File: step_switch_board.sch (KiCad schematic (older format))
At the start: 37 parts

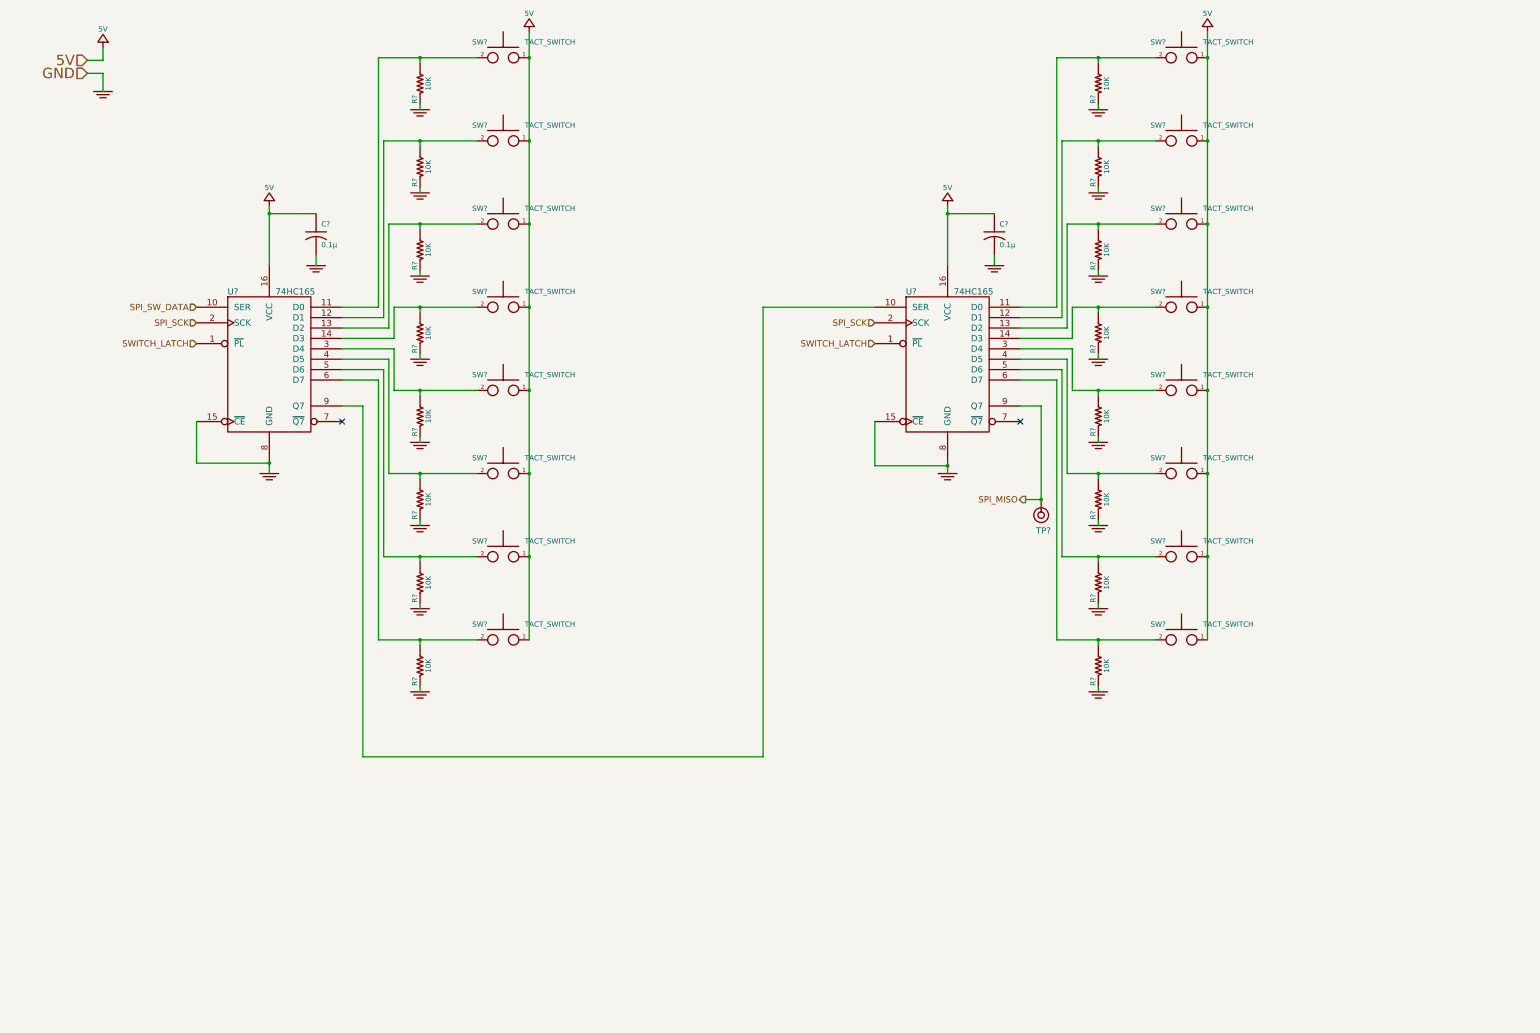
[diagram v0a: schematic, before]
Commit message: more SPI work
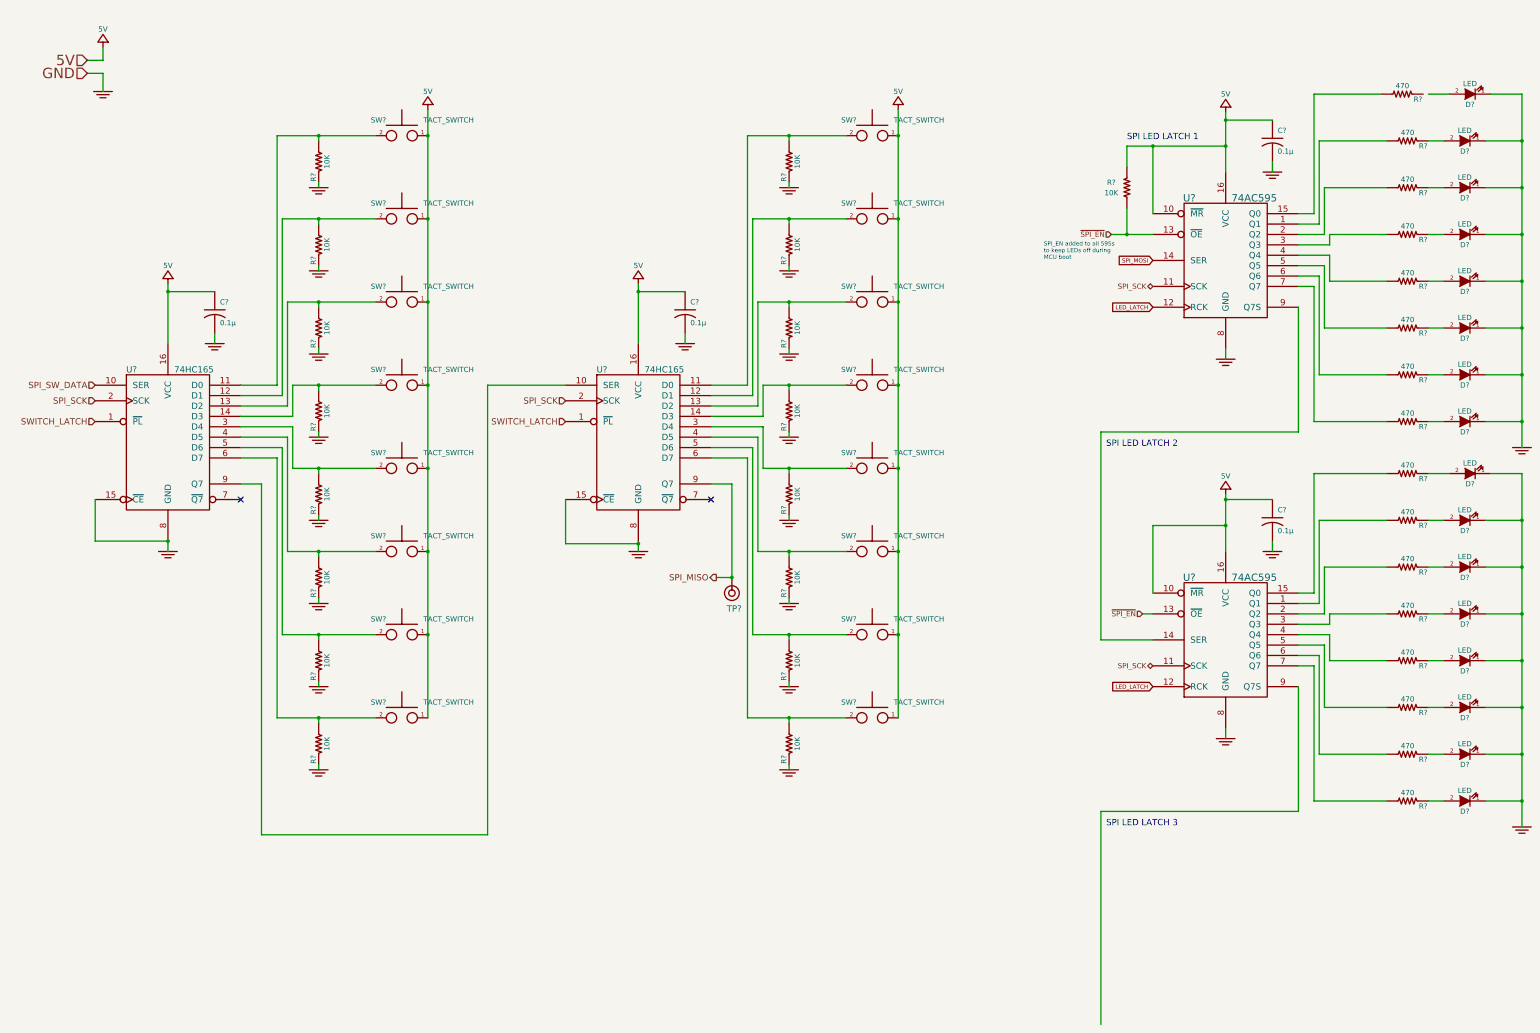
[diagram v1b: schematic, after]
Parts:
- added C? (x2): 0.1µ, ~, symbol C_US
- added D? (x16): LED, symbol LED
- added R?: 10K, ~, symbol R_US
- added R? (x16): 470, ~, symbol R_US
- added U? (x2): 74AC595, symbol 74AC595
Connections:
- net +5V: now also C?.1, C?.1, R?.1, U?.10 (~MR), U?.10 (~MR), U?.16 (VCC), U?.16 (VCC)
- net GND: now also C?.2, C?.2, D?.1 (K), D?.1 (K), D?.1 (K), D?.1 (K), D?.1 (K), D?.1 (K), D?.1 (K), D?.1 (K), D?.1 (K), D?.1 (K), D?.1 (K), D?.1 (K), D?.1 (K), D?.1 (K), D?.1 (K), D?.1 (K), U?.8 (GND), U?.8 (GND)
- net SPI_SCK: now also U?.11 (SCK), U?.11 (SCK)
- new net: D?.2 (A), R?.1 (x15)
- new net: R?.2, U?.2 (Q2) (x2)
- new net: R?.2, U?.1 (Q1) (x2)
- new net: R?.2, U?.5 (Q5) (x2)
- new net: R?.2, U?.4 (Q4) (x2)
- new net: R?.2, U?.3 (Q3) (x2)
- new net: R?.2, U?.15 (Q0) (x2)
- new net: R?.2, U?.6 (Q6) (x2)
- new net: R?.2, U?.7 (Q7) (x2)
- new net: U?.14 (SER), U?.9 (Q7S)
- new net LED_LATCH: U?.12 (RCK), U?.12 (RCK)
- new net SPI_MOSI: U?.14 (SER)
- new net ~SPI_EN: R?.2, U?.13 (~OE), U?.13 (~OE)
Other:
- note added: "SPI LED LATCH 1"
- note added: "SPI LED LATCH 2"
- note added: "SPI LED LATCH 3"
- note added: "SPI_EN added to all 595s\nto keep LEDs off during\nMCU boot"
- moved on the sheet: C?, R?, SW?, TP?, U?
